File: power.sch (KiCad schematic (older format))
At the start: 59 parts, among them U1 TPS2420, U2 LT3487, U3 TPS63002, U4 LM3674, U5 TPS56x200, U6 TPS56x200, U7 TPS56x200, U8 LMZ10500

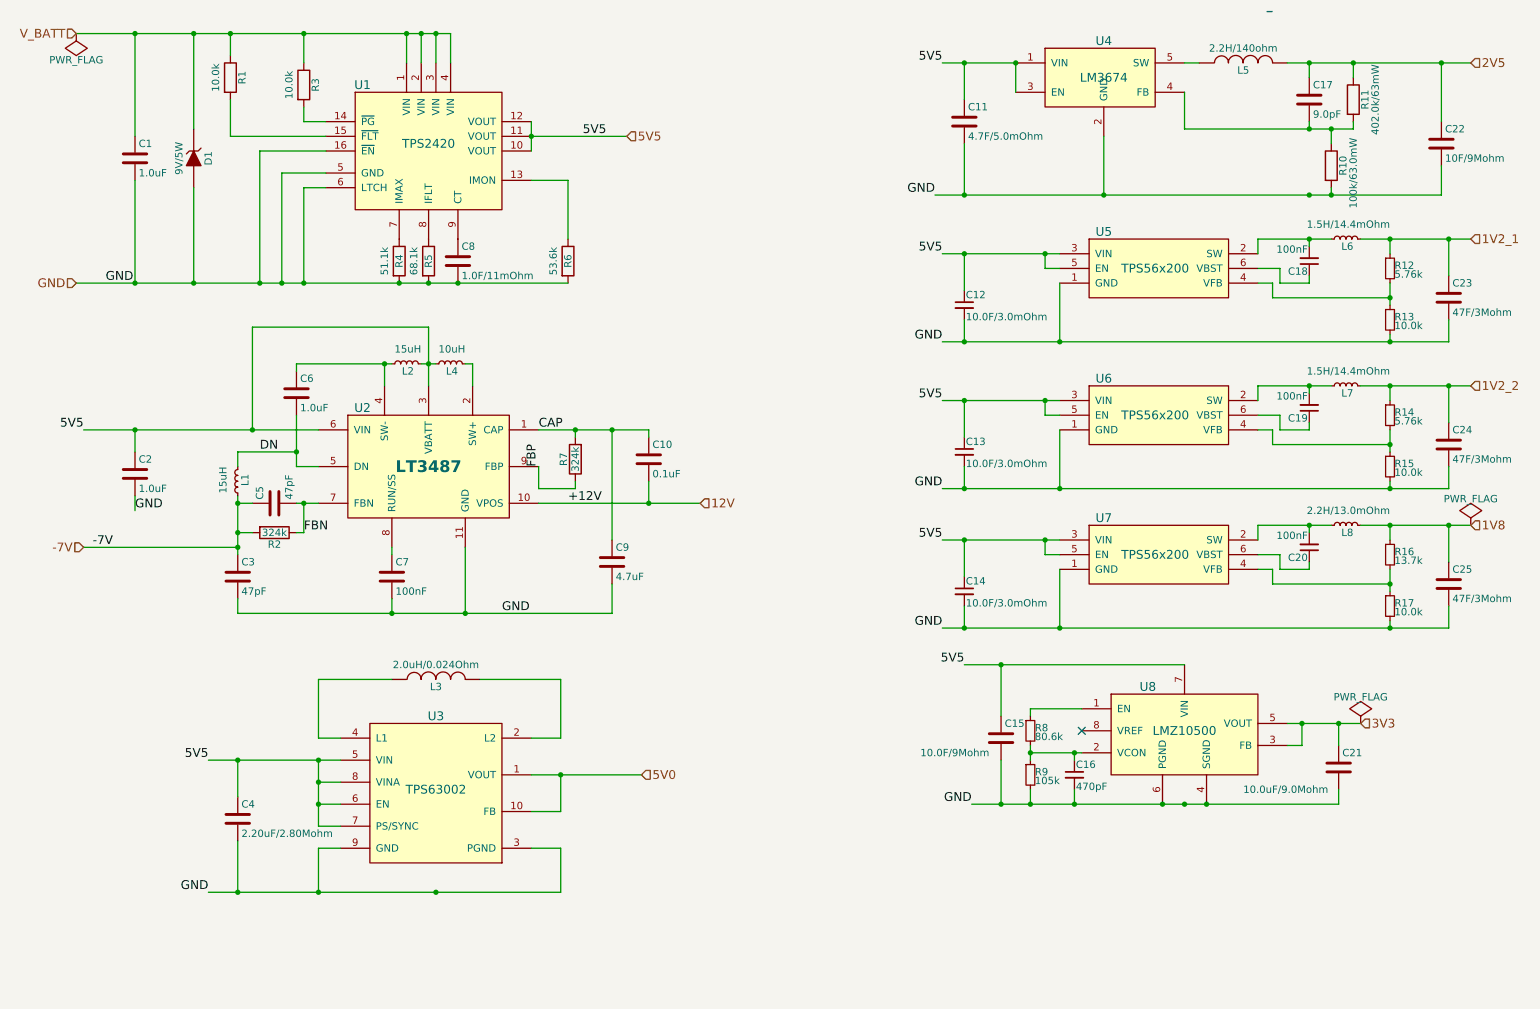
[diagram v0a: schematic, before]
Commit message: Lot's of back and forward with vendor.
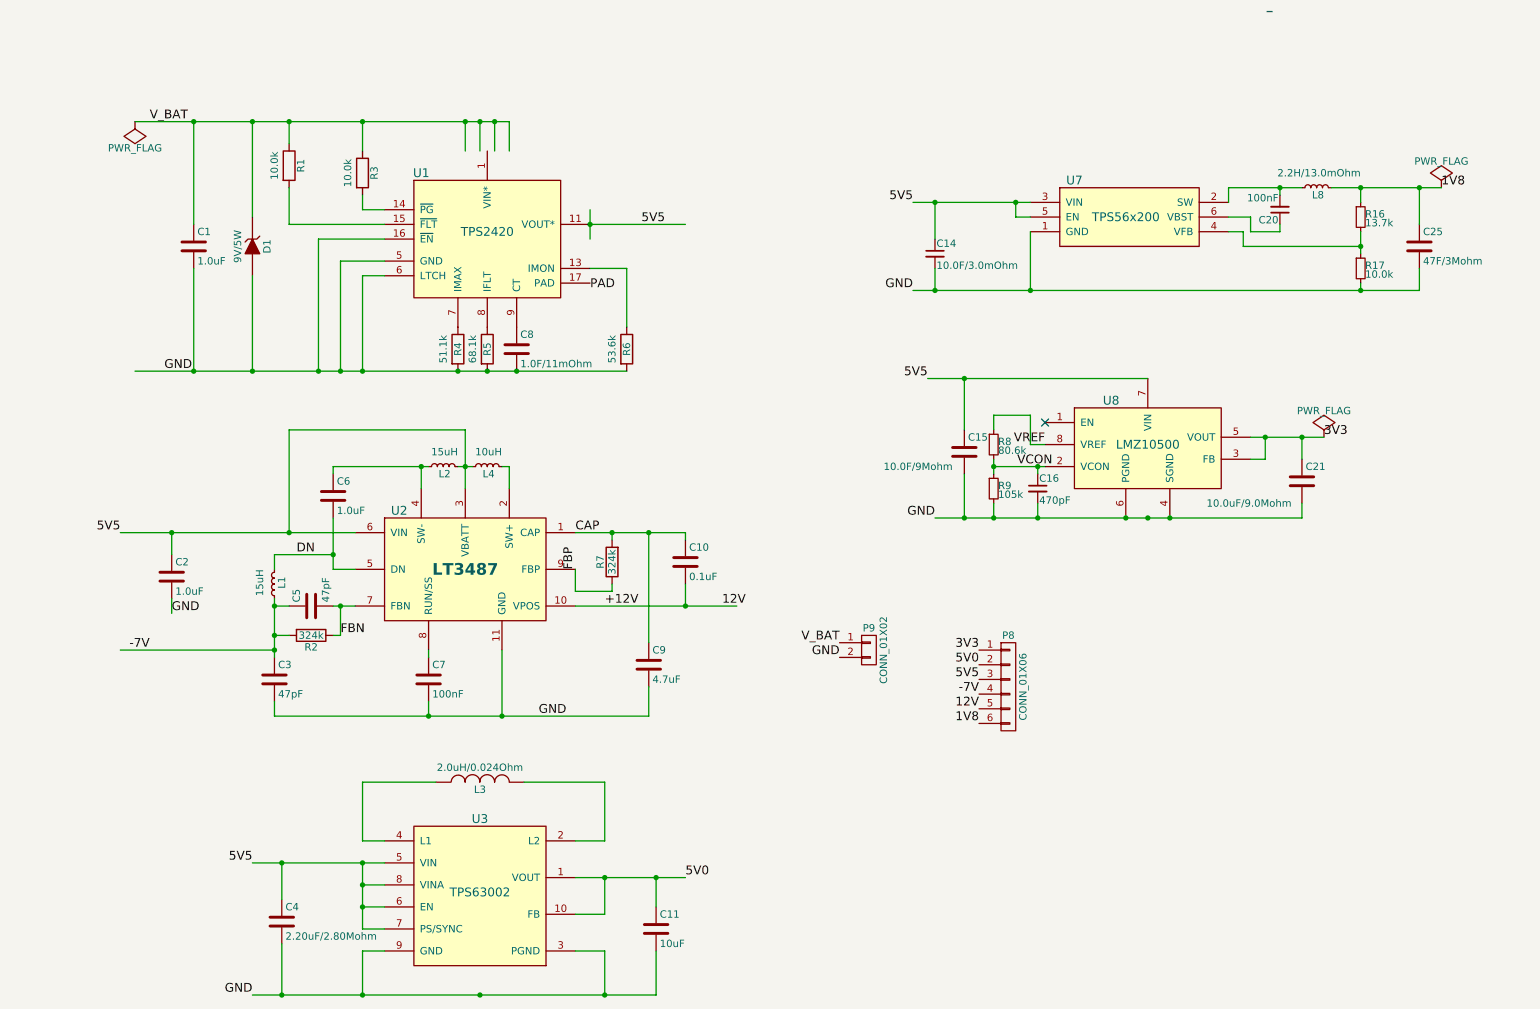
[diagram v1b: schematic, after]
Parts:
- removed C12, C13: 10.0F/3.0mOhm, w_smd_cap:c_0603, symbol C_Small
- removed C17: 9.0pF, Capacitors_SMD:C_0805_HandSoldering, symbol C
- removed C18, C19: 100nF, w_smd_cap:c_0603, symbol C_Small
- removed C22: 10F/9Mohm, Capacitors_SMD:C_0603_HandSoldering, symbol C
- removed C23, C24: 47F/3Mohm, w_smd_cap:c_0603, symbol C
- removed L5: 2.2H/140ohm, camera:Inductor_SMD_2016, symbol INDUCTOR
- removed L6, L7: 1.5H/14.4mOhm, w_smd_inductors:inductor_smd_0805, symbol L_Small
- removed R10: 100k/63.0mW, Resistors_SMD:R_0402, symbol R
- removed R11: 402.0k/63mW, Resistors_SMD:R_0402, symbol R
- removed R12, R14: 5.76k, w_smd_resistors:r_0805, symbol R_Small
- removed R13, R15: 10.0k, w_smd_resistors:r_0805, symbol R_Small
- removed U1: TPS2420, Housings_DFN_QFN:QFN-16-1EP_4x4mm_Pitch0.65mm, symbol TPS2420-RESCUE-AstroCam
- removed U4: LM3674, w_smd_trans:sot23-5, symbol LM3674
- removed U5, U6: TPS56x200, w_smd_trans:sot23-6, symbol TPS56x200
- added P8: CONN_01X06, w_pin_strip:pin_socket_6, symbol CONN_01X06
- added P9: CONN_01X02, w_pin_strip:pin_socket_2, symbol CONN_01X02
- added U1: TPS2420, camera:S-PVQFN-N16, symbol TPS2420
- C11: value 4.7F/5.0mOhm -> 10uF; footprint Capacitors_SMD:C_0603_HandSoldering -> Capacitors_SMD:C_0805_HandSoldering; Component (none) -> TDK C1608X5R1A105K
- U3: footprint (none) -> Housings_DFN_QFN:DFN-10-1EP_3x3mm_Pitch0.5mm
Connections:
- net labels added: PAD, VCON, VREF, V_BAT
- net labels removed: 1V2_1, 1V2_2, 2V5, V_BATT
- wire segments 193 -> 132
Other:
- moved on the sheet: C1, C10, C14, C15, C16, C2, C20, C21, C25, C3, C4, C5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
